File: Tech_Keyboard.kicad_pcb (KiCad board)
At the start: 2 copper layers, 35 parts, among them U1 MCU_Seeed_XIAO_RP2040

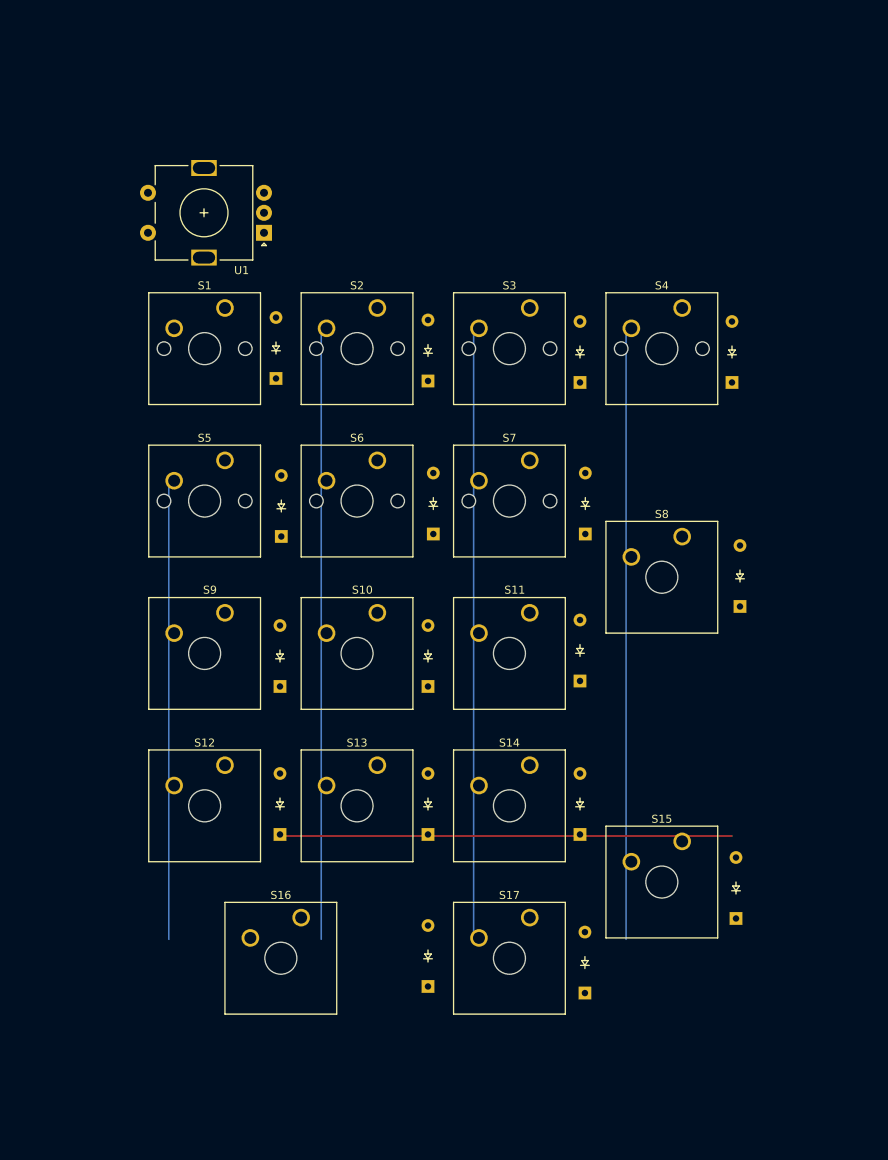
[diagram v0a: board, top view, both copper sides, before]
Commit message: wiring done
wired up pcb and fixed schematic... kind mad cuz i spent 3 hours and forgot to hit record...
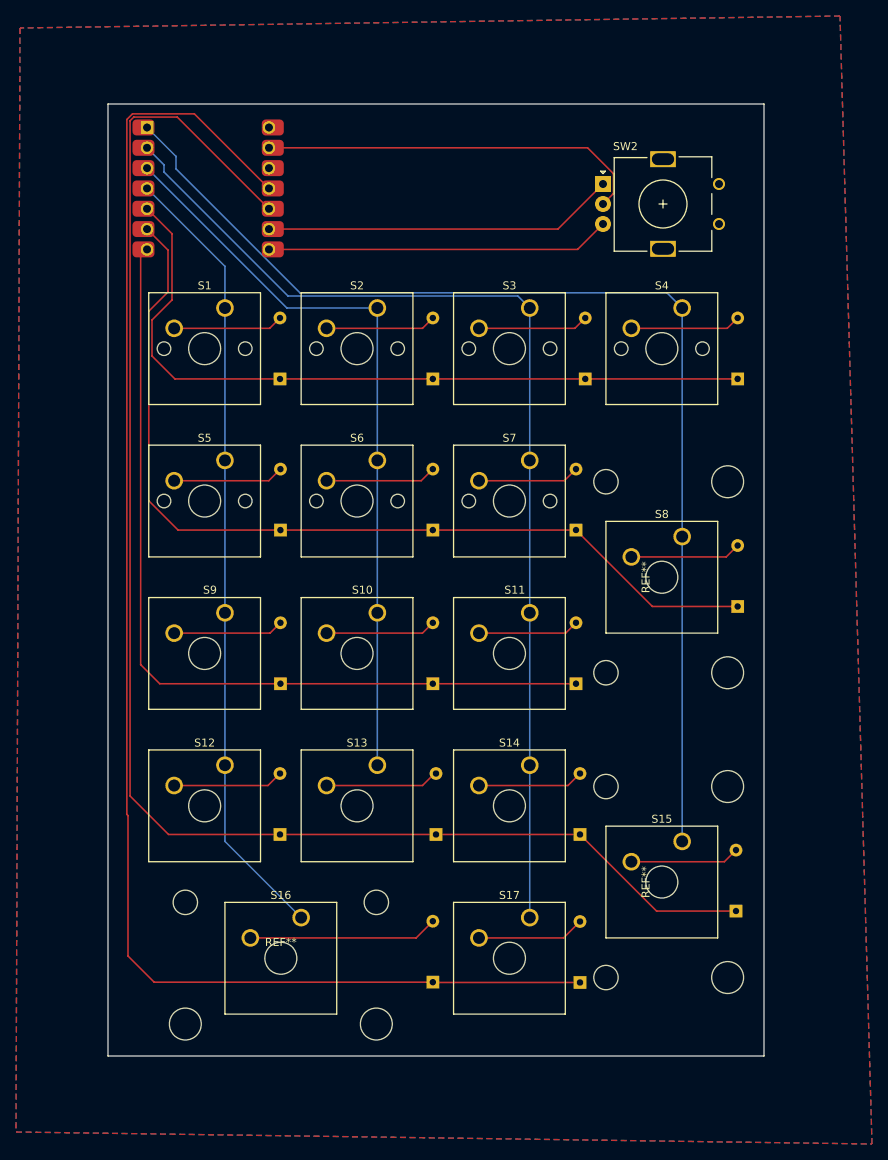
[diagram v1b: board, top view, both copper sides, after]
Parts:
- added REF**: Stabilizer_MX_2.00u, ScottoKeebs_Stabilizer:Stabilizer_MX_2.00u, F.Cu at (180.2, 135.8)
- added REF**: Stabilizer_MX_2.00u, ScottoKeebs_Stabilizer:Stabilizer_MX_2.00u, F.Cu at (180.2, 97.7)
- added REF**: Stabilizer_MX_2.00u, ScottoKeebs_Stabilizer:Stabilizer_MX_2.00u, F.Cu at (132.6, 145.3)
- added SW2: RotaryEncoder, Rotary_Encoder:RotaryEncoder_Alps_EC11E_Vertical_H20mm, F.Cu at (172.9, 48.5)
- D1, D10, D11, D12, D13, D14, D15, D16, D17, D2, D3, D4, D5, D6, D7, D8, D9: moved to B.Cu
- U1: footprint Rotary_Encoder:RotaryEncoder_Alps_EC11E-Switch_Vertical_H20mm -> ScottoKeebs_MCU:Seeed_XIAO_RP2040
- moved U1 8.93 mm to (123.5, 49.1), turned to 0 degrees
- moved D17 1.46 mm to (170.0, 148.3)
- moved D7 1.26 mm to (169.5, 91.8)
- moved D13 1.00 mm to (152.0, 129.8)
- moved D15 0.93 mm to (189.5, 139.4)
- moved D4 0.83 mm to (189.7, 72.9)
- moved D16 0.81 mm to (151.6, 148.3)
- moved D5 0.81 mm to (132.6, 91.8)
- moved D3 0.79 mm to (170.7, 72.9)
- moved D10 0.70 mm to (151.6, 111.0)
- moved D2 0.66 mm to (151.6, 72.9)
- moved D11 0.61 mm to (169.5, 111.0)
- moved D1 0.50 mm to (132.5, 72.9)
- moved D6 0.50 mm to (151.6, 91.8)
- moved D9 0.35 mm to (132.6, 111.0)
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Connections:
- D1 pad 1: Column 0 -> Row 0
- D1 pad 2: Column 0 -> Row 0
- D10 pad 1: Column 0 -> Row 2
- D10 pad 2: Column 0 -> Row 2
- D11 pad 1: Column 0 -> Row 2
- D11 pad 2: Column 0 -> Row 2
- D12 pad 1: Column 0 -> Row 3
- D12 pad 2: Column 0 -> Row 3
- D13 pad 1: Column 0 -> Row 3
- D13 pad 2: Column 0 -> Row 3
- D14 pad 1: Column 0 -> Row 3
- D14 pad 2: Column 0 -> Row 3
- D15 pad 1: Column 0 -> Row 3
- D15 pad 2: Column 0 -> Row 3
- D16 pad 1: Column 0 -> Row 4
- D16 pad 2: Column 0 -> Row 4
- D17 pad 1: Column 0 -> Row 4
- D17 pad 2: Column 0 -> Row 4
- D2 pad 1: Column 0 -> Row 0
- D2 pad 2: Column 0 -> Row 0
- D3 pad 1: Column 0 -> Row 0
- D3 pad 2: Column 0 -> Row 0
- D4 pad 1: Column 0 -> Row 0
- D4 pad 2: Column 0 -> Row 0
- D5 pad 1: Column 0 -> Row 1
- D5 pad 2: Column 0 -> Row 1
- D6 pad 1: Column 0 -> Row 1
- D6 pad 2: Column 0 -> Row 1
- D7 pad 1: Column 0 -> Row 1
- D7 pad 2: Column 0 -> Row 1
- D8 pad 1: Column 0 -> Row 1
- D8 pad 2: Column 0 -> Row 1
- D9 pad 1: Column 0 -> Row 2
- D9 pad 2: Column 0 -> Row 2
- S1 pad 1: (no net) -> Column 0
- S1 pad 2: (no net) -> Row 0
- S10 pad 1: Column 0 -> Column 1
- S10 pad 2: Column 0 -> Row 2
- S11 pad 1: Column 0 -> Column 2
- S11 pad 2: Column 0 -> Row 2
- S12 pad 2: Column 0 -> Row 3
- S13 pad 1: Column 0 -> Column 1
- S13 pad 2: Column 0 -> Row 3
- S14 pad 1: Column 0 -> Column 2
- S14 pad 2: Column 0 -> Row 3
- S15 pad 1: Column 0 -> Column 3
- S15 pad 2: Column 0 -> Row 3
- S16 pad 2: Column 0 -> Row 4
- S17 pad 1: Column 0 -> Column 2
- S17 pad 2: Column 0 -> Row 4
- S2 pad 1: Column 0 -> Column 1
- S2 pad 2: Column 0 -> Row 0
- S3 pad 1: Column 0 -> Column 2
- S3 pad 2: Column 0 -> Row 0
- S4 pad 1: Column 0 -> Column 3
- S4 pad 2: Column 0 -> Row 0
- S5 pad 2: Column 0 -> Row 1
- S6 pad 1: Column 0 -> Column 1
- S6 pad 2: Column 0 -> Row 1
- S7 pad 1: Column 0 -> Column 2
- S7 pad 2: Column 0 -> Row 1
- S8 pad 1: Column 0 -> Column 3
- S8 pad 2: Column 0 -> Row 1
- S9 pad 2: Column 0 -> Row 2
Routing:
- net Column 0: track 343.1 -> 99.1 mm
- net Row 3: track 0.00 -> 243.0 mm
- net Row 4: track 0.00 -> 221.6 mm
- net Row 1: track 0.00 -> 169.7 mm
- net Row 0: track 0.00 -> 150.4 mm
- net Row 2: track 0.00 -> 148.0 mm
- net Column 3: track 0.00 -> 143.8 mm
- net Column 2: track 0.00 -> 132.9 mm
- net Column 1: track 0.00 -> 93.2 mm
- net GND: track 0.00 -> 48.3 mm
- net R0: track 0.00 -> 44.1 mm
- net R1: track 0.00 -> 43.1 mm
- added copper zone on B.Cu, net (none)
- added copper zone on F.Cu, net (none)
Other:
- board outline added: 82 x 119 mm
